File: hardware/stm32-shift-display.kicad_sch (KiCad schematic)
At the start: 43 parts, among them J1 HDR_SWD, J2 USB_C_Receptacle_USB2.0_16P, SW1 SW_PUSH, SW2 SW_PUSH, SW3 SW_PUSH, SW4 SW_PUSH, SW5 218-2LPSTR, U1 AMS1117-3.3, U2 STM32F103C8T6, X1 OT32258MJBA4SL, X2 OK322532.768KJBA4SL

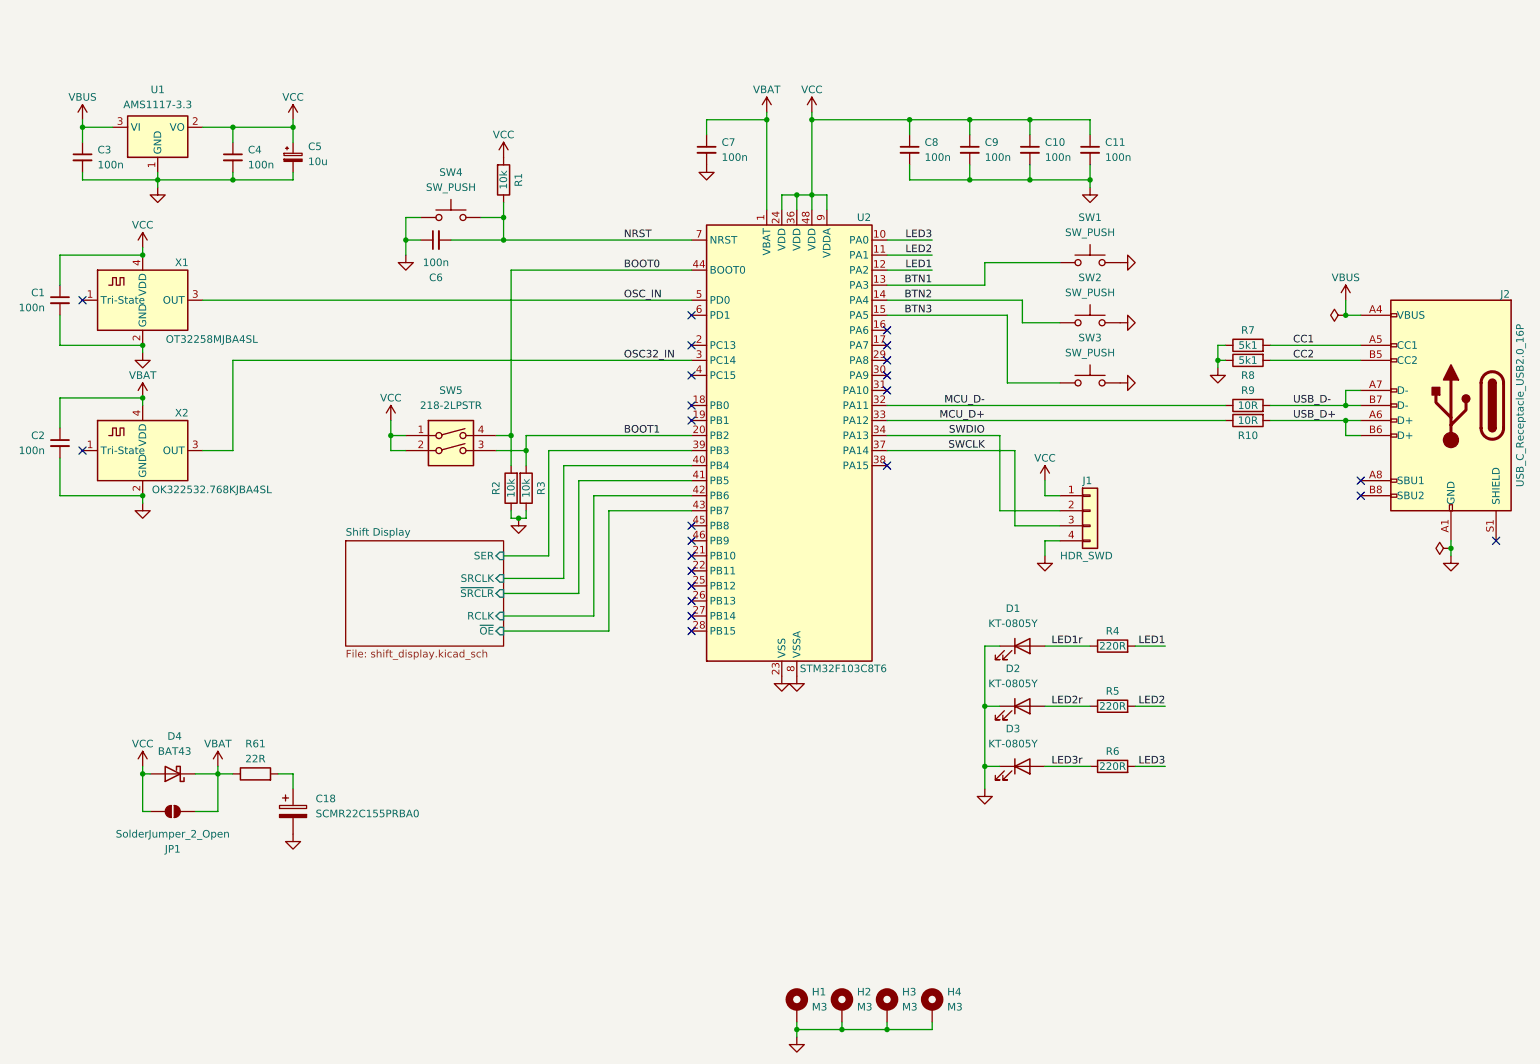
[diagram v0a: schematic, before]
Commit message: update readme
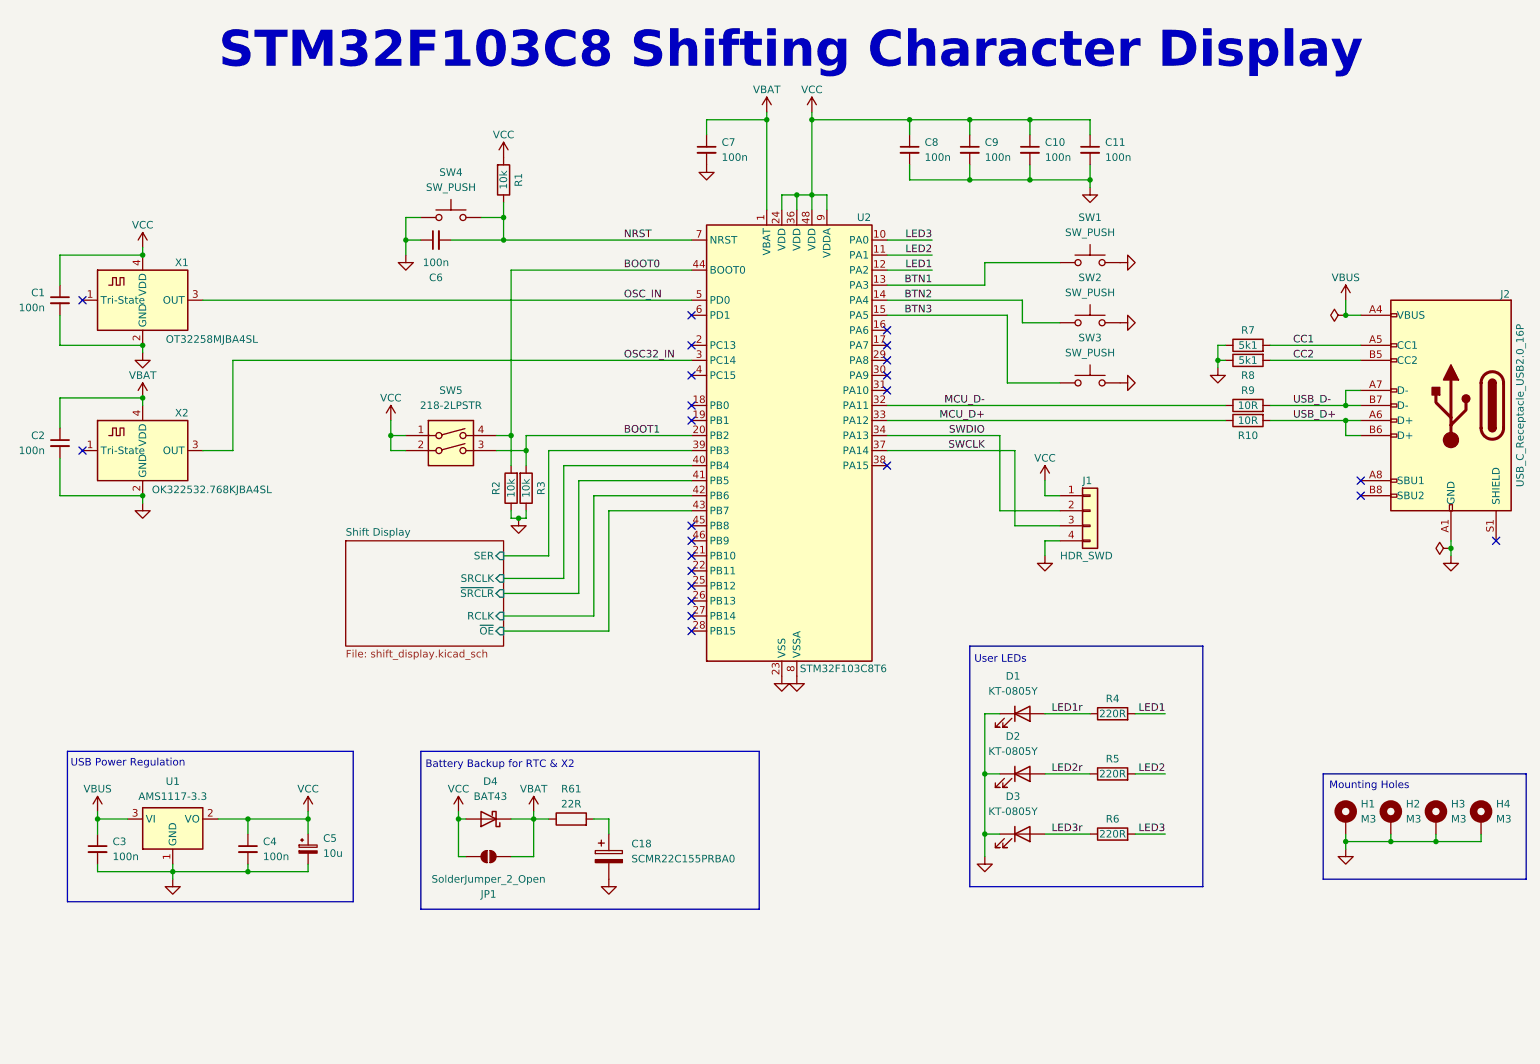
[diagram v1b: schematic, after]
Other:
- note added: "Battery Backup for RTC & X2"
- note added: "Mounting Holes"
- note added: "STM32F103C8 Shifting Character Display"
- note added: "USB Power Regulation"
- note added: "User LEDs"
- moved on the sheet: C18, C3, C4, C5, D1, D2, D3, D4, H1, H2, H3, H4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
